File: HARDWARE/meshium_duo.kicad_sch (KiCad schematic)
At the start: 12 parts, among them J7 Conn_01x02_Pin, J8 Conn_02x03_Odd_Even

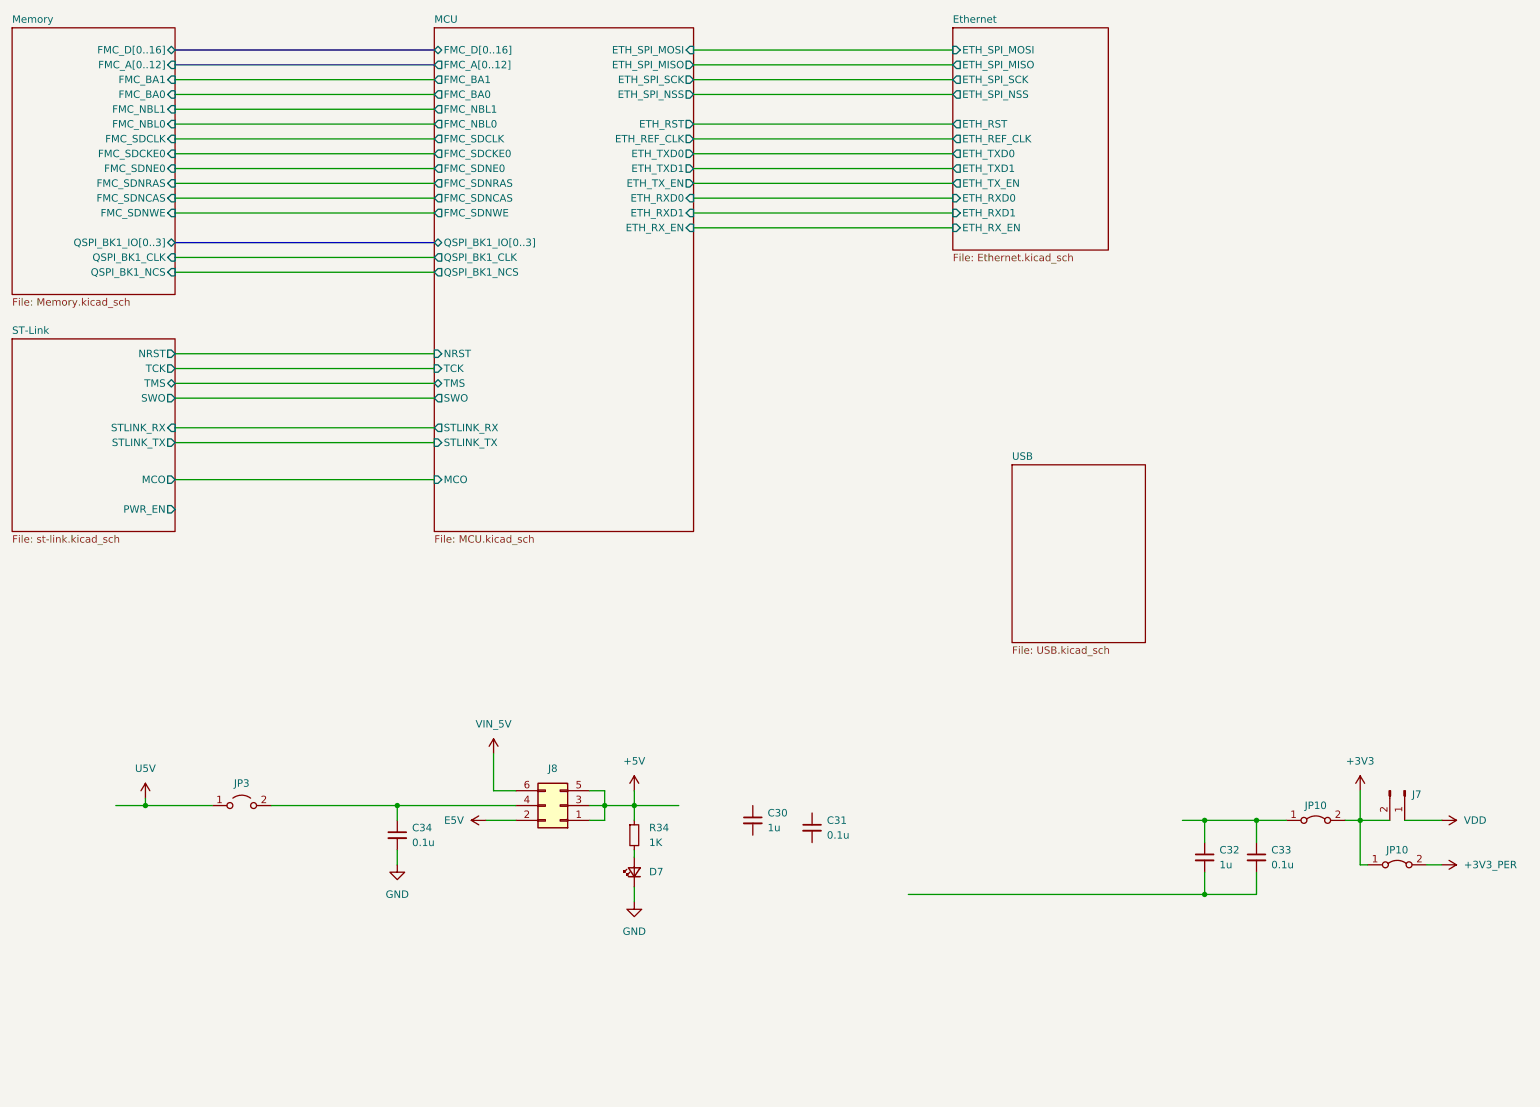
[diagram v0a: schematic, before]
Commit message: schematic capture
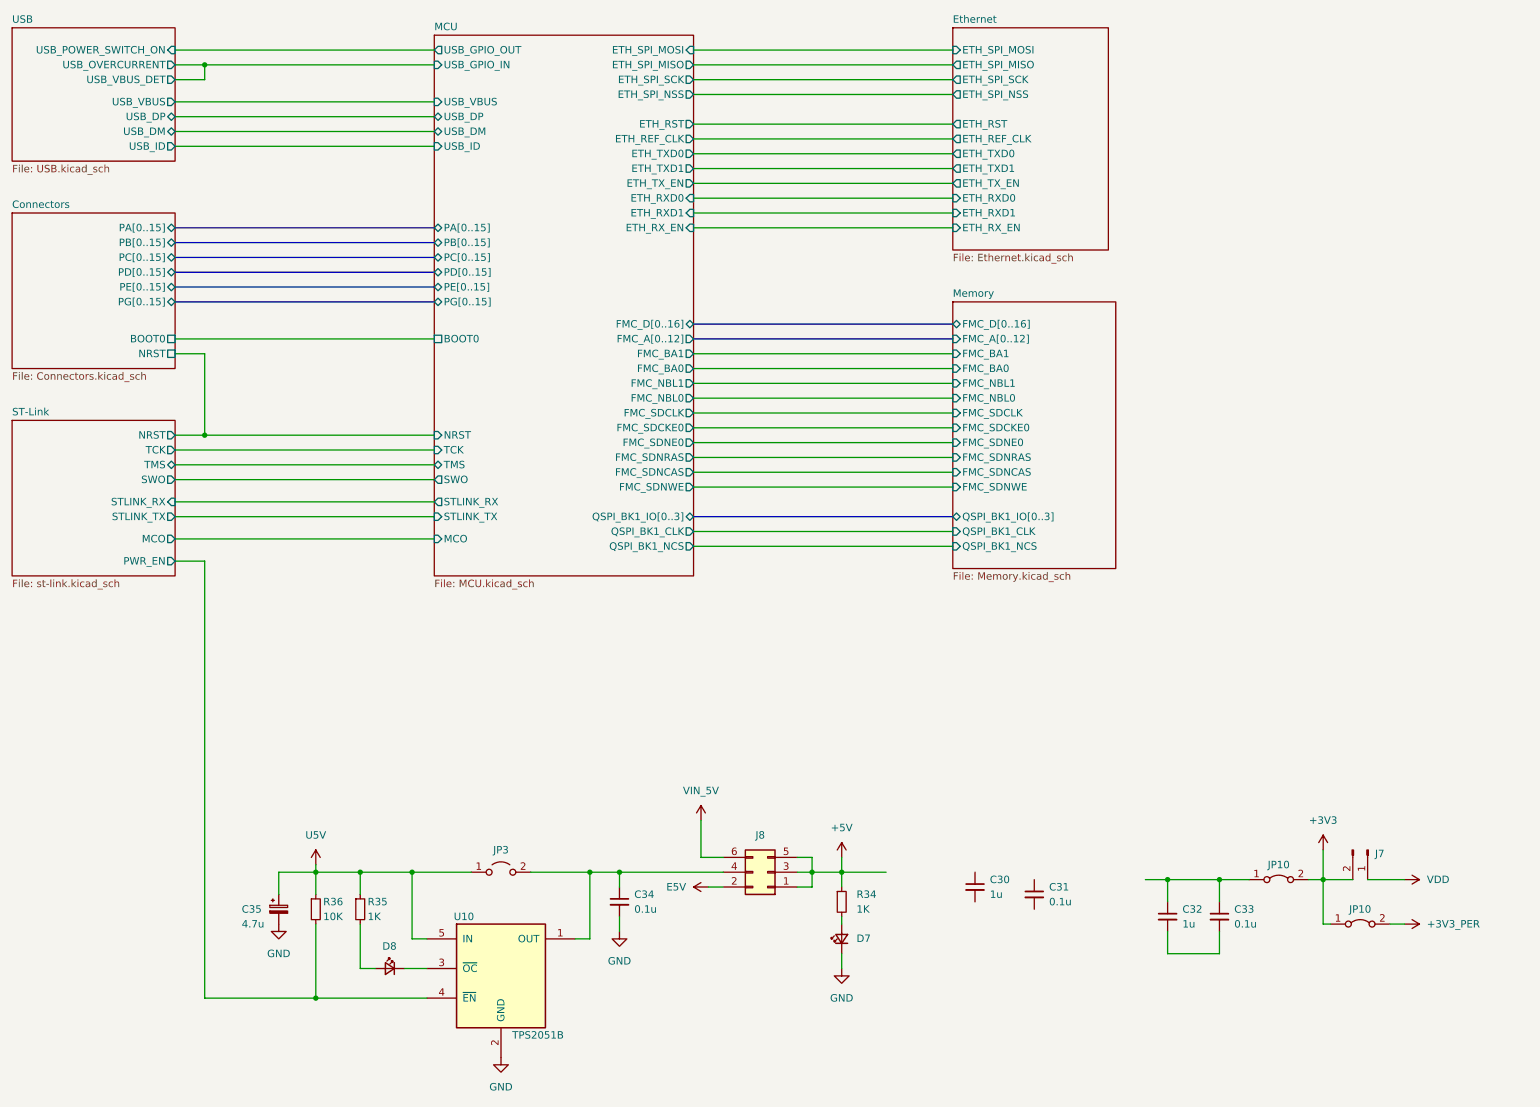
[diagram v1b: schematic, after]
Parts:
- added C35: 4.7u, Capacitor_Tantalum_SMD:CP_EIA-6032-28_Kemet-C, symbol Device:C_Polarized_Small
- added D8: LED_Small, LED_SMD:LED_0603_1608Metric, symbol Device:LED_Small
- added R35: 1K, Resistor_SMD:R_0603_1608Metric, symbol Device:R_Small
- added R36: 10K, Resistor_SMD:R_0603_1608Metric, symbol Device:R_Small
- added U10: TPS2051B, Package_TO_SOT_SMD:SOT-23-5, symbol meshium_duo:TPS2051B
- D7: footprint (none) -> LED_SMD:LED_0603_1608Metric
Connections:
- net +5V0: now also C35.1, R35.1, R36.1, U10.5 (IN)
- net GND: now also C35.2, U10.2 (GND)
- net ST-Link/PWR_EN: now also R36.2, U10.4 (~{EN})
- net at C34.1, J8.4 (Pin_4), JP3.2 (B): now also U10.1 (OUT)
- new net: D8.1 (K), U10.3 (~{OC})
- new net: D8.2 (A), R35.2
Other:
- added sheet Connectors (Connectors.kicad_sch)
- sheet MCU ports: added BOOT0, PA[0..15], PB[0..15], PC[0..15], PD[0..15], PE[0..15], PG[0..15], USB_DM, USB_DP, USB_GPIO_IN, USB_GPIO_OUT, USB_ID, USB_VBUS; removed none
- sheet USB ports: added USB_DM, USB_DP, USB_ID, USB_OVERCURRENT, USB_POWER_SWITCH_ON, USB_VBUS, USB_VBUS_DET; removed none
- moved on the sheet: C30, C31, C32, C33, C34, D7, J7, J8, JP10, JP3, R34
